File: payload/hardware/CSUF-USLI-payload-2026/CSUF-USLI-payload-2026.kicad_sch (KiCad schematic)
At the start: 21 parts, among them U1 DEV-16771, U2 GPS6MV2, U3 MPU6050, U4 Adafruit BMP280, U5 RYLR896, U6 Generic RS485 to UART, U7 DF Robot EC and pH Placeholder

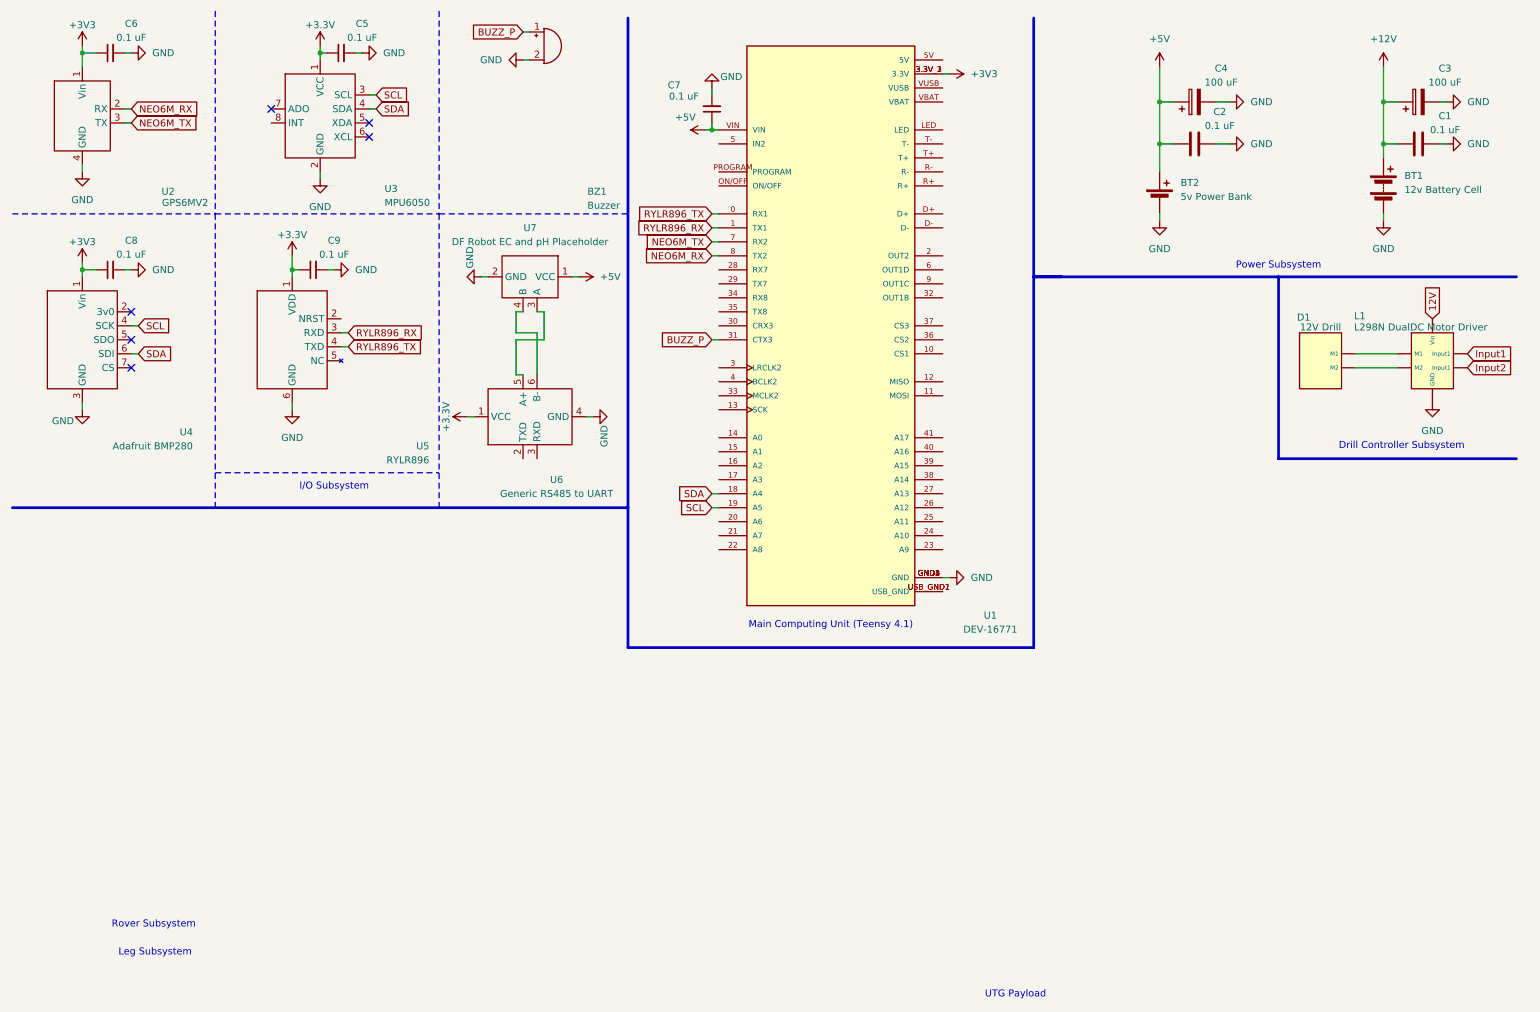
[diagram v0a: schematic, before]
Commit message: idk what change i did
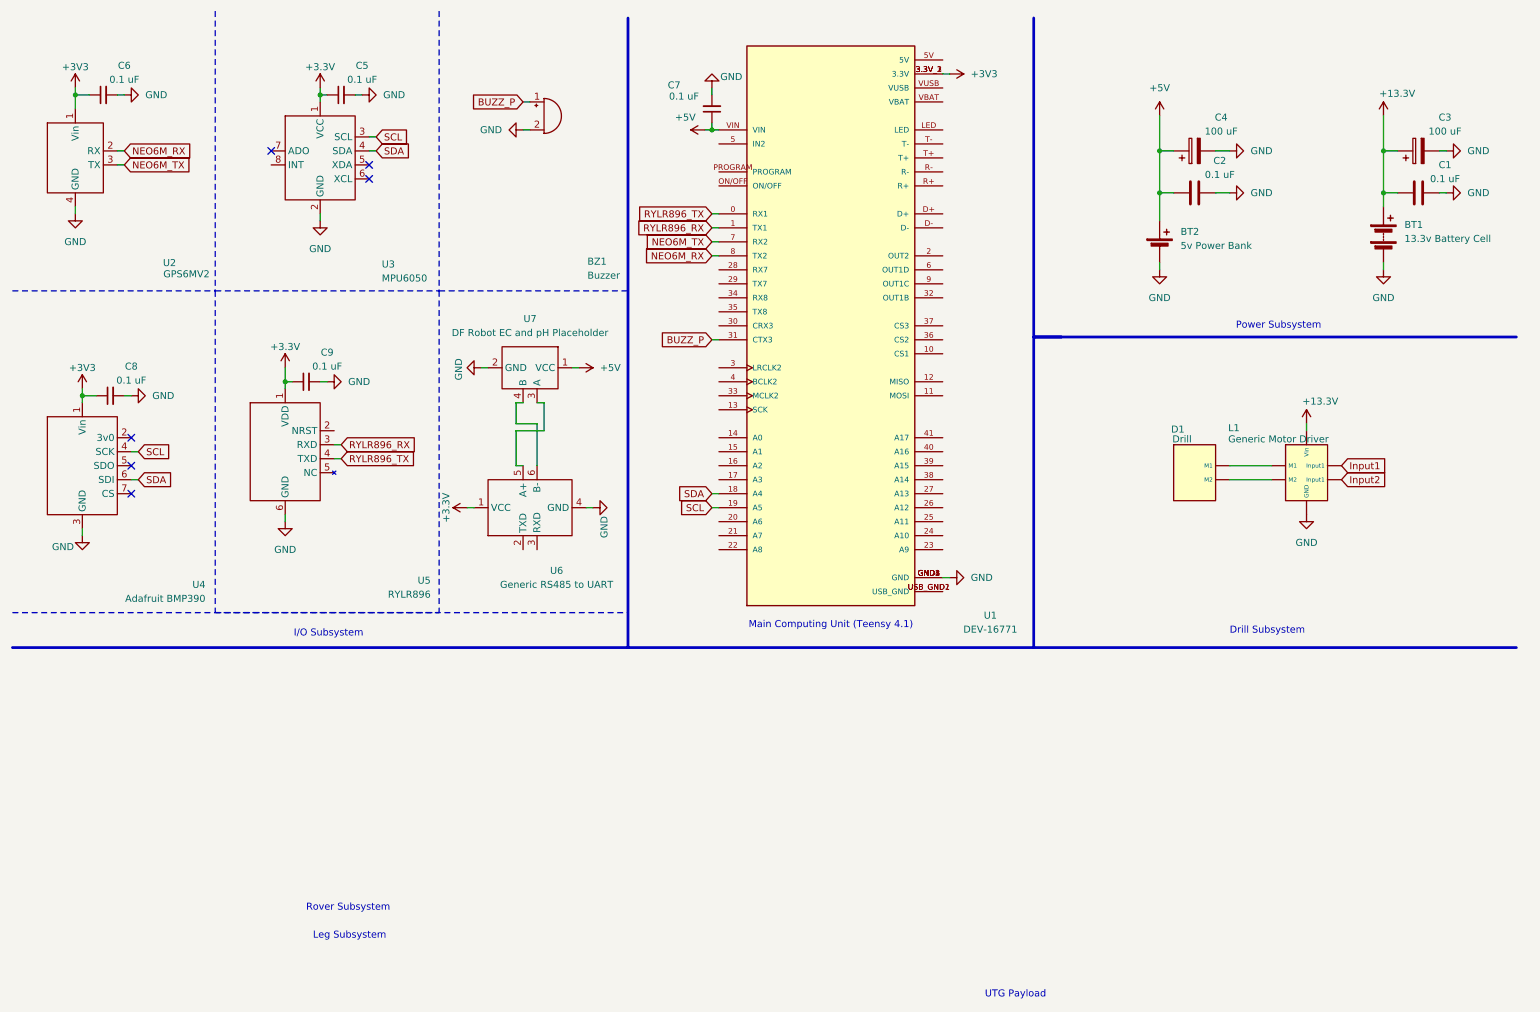
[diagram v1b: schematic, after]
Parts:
- BT1: value 12v Battery Cell -> 13.3v Battery Cell
- D1: value 12V Drill -> Drill
- L1: value L298N DualDC Motor Driver -> Generic Motor Driver
- U4: value Adafruit BMP280 -> Adafruit BMP390
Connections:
- net 12V is gone; now on net Input2: L1. (Input1)
- net +12V renamed +13.3V
- net +13.3V: now also L1. (Input1)
- new net: D1. (M2), L1. (Input1)
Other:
- note added: "Drill Subsystem"
- note removed: "Drill Controller Subsystem"
- moved on the sheet: BT1, BT2, BZ1, C1, C2, C3, C4, C5, C6, C8, C9, D1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
